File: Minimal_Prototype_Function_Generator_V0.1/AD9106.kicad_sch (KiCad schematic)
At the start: 30 parts, among them IC1 AD9106BCPZ, J1 142-0701-201, Y1 AX3DCF1-156.2500T

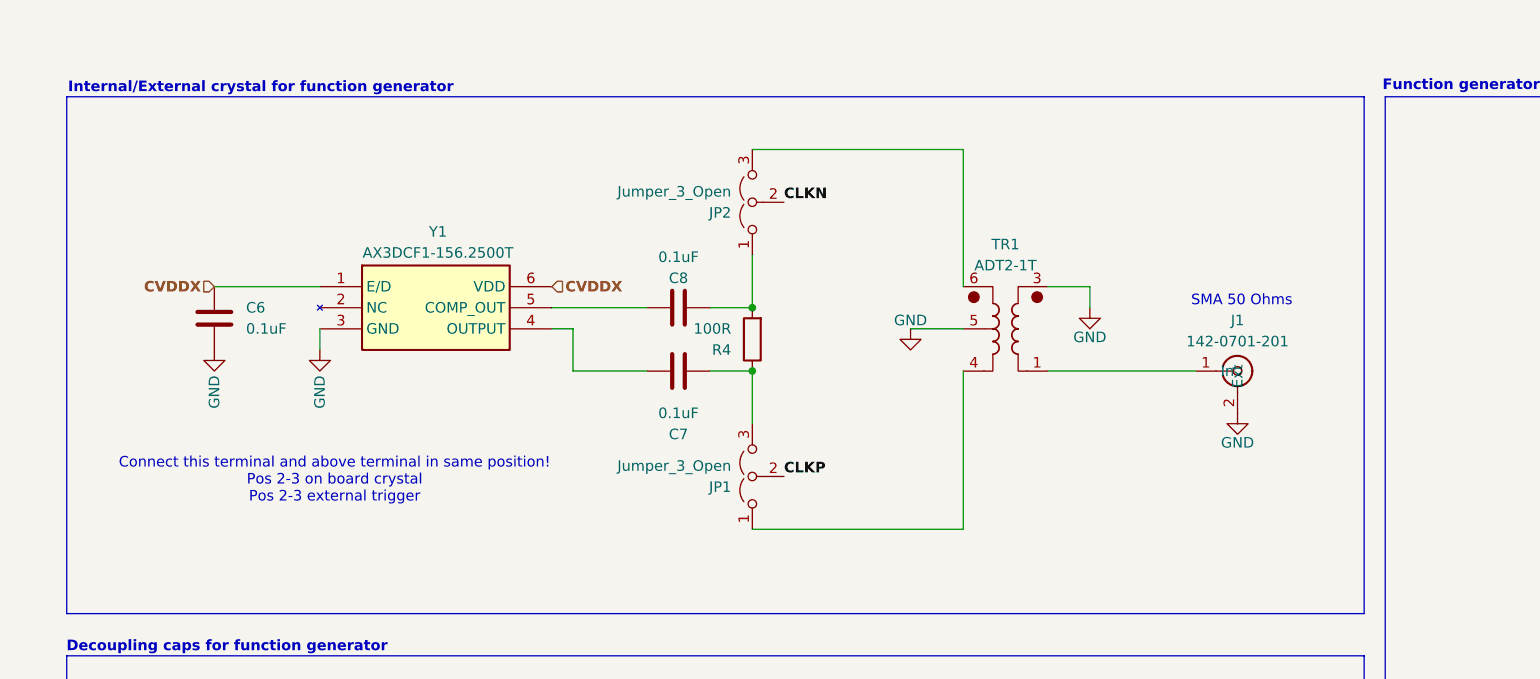
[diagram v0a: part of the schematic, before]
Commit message: Routing PCB, not yet finished
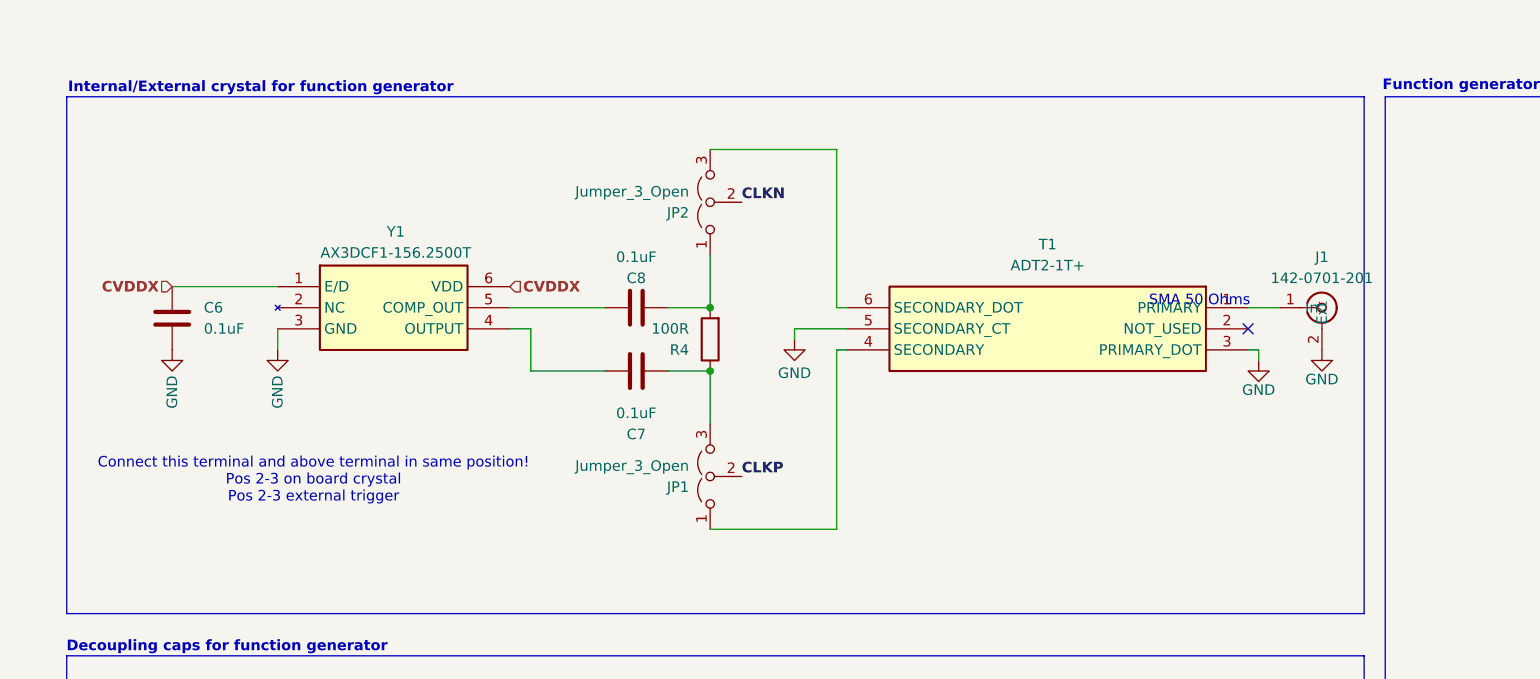
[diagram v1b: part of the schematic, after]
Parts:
- removed TR1: ADT2-1T, RF_Mini-Circuits:Mini-Circuits_CD542_H2.84mm, symbol Transformer:ADT2-1T
- added T1: ADT2-1T+, Insyte_Footprints:ADT21T, symbol ADT2-1T+:ADT2-1T+
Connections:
- net GND: now also T1.3 (PRIMARY_DOT), T1.5 (SECONDARY_CT)
- net at J1.1 (In): now also T1.1 (PRIMARY)
- net at JP1.1 (A): now also T1.4 (SECONDARY)
- net at JP2.3 (B): now also T1.6 (SECONDARY_DOT)
- no-connect marks 0 -> 1
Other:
- moved on the sheet: C6, C7, C8, J1, JP1, JP2, R4, Y1
